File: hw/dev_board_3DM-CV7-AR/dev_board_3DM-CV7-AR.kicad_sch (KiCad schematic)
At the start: 26 parts, among them J1 87438-0643, U1 DMP2240UW, U2 DMP2240UW

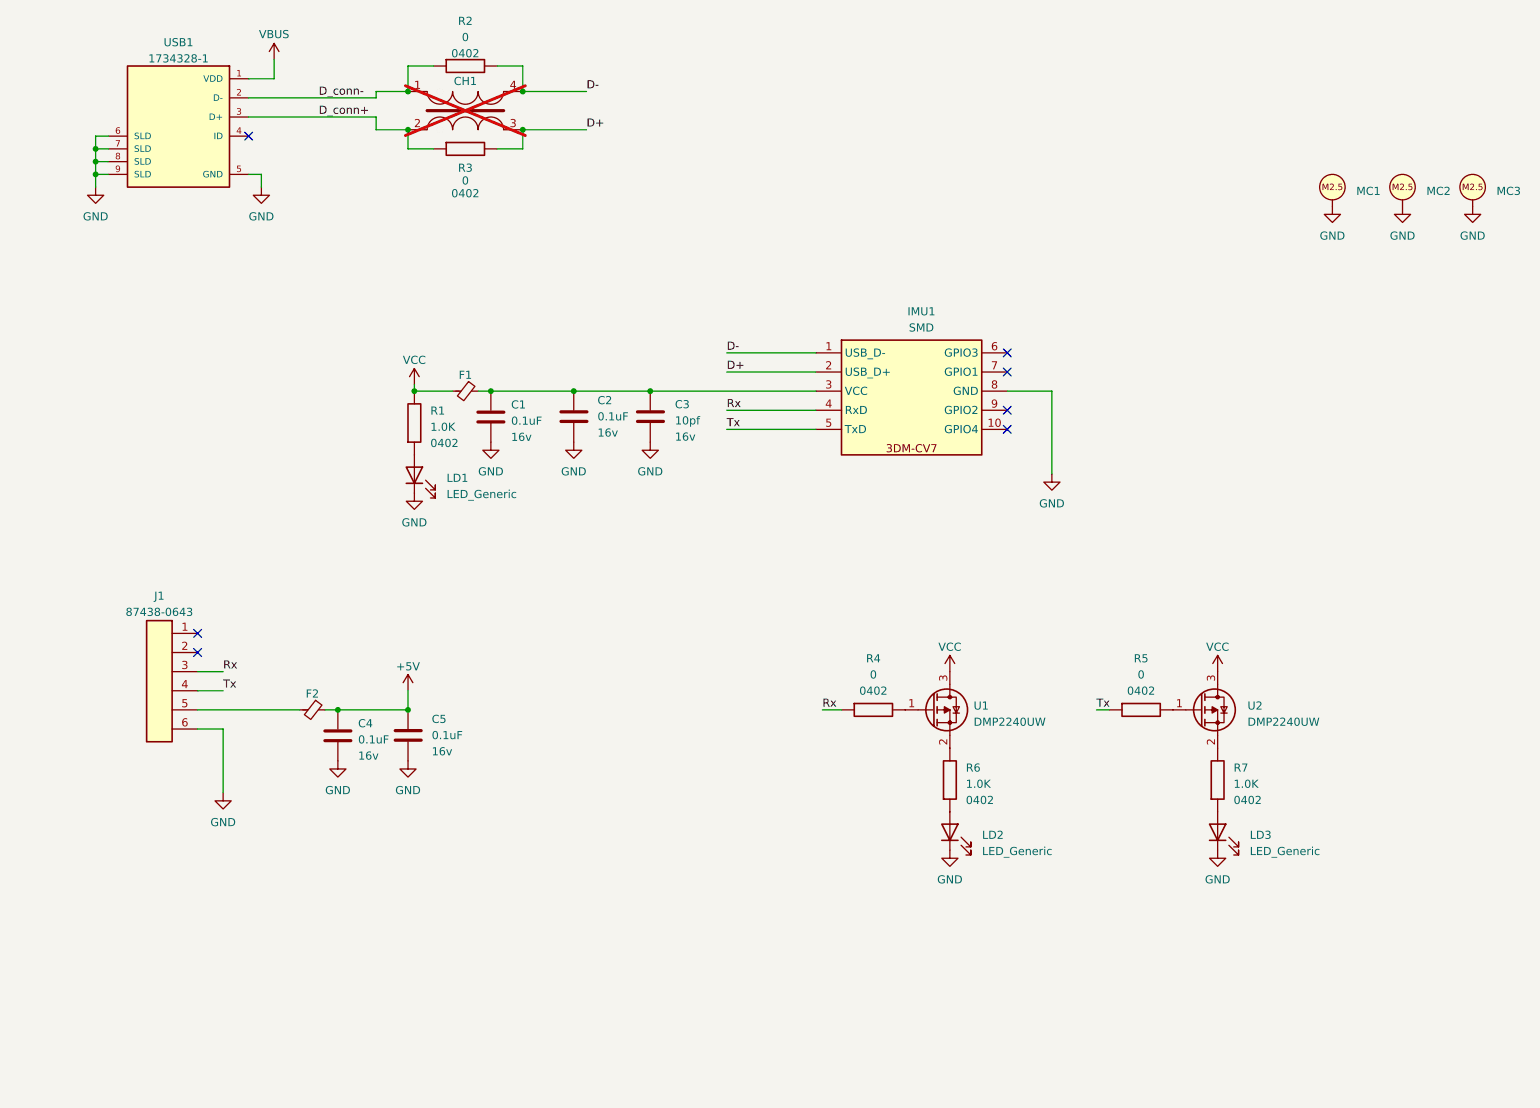
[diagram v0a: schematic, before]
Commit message: Finalizado
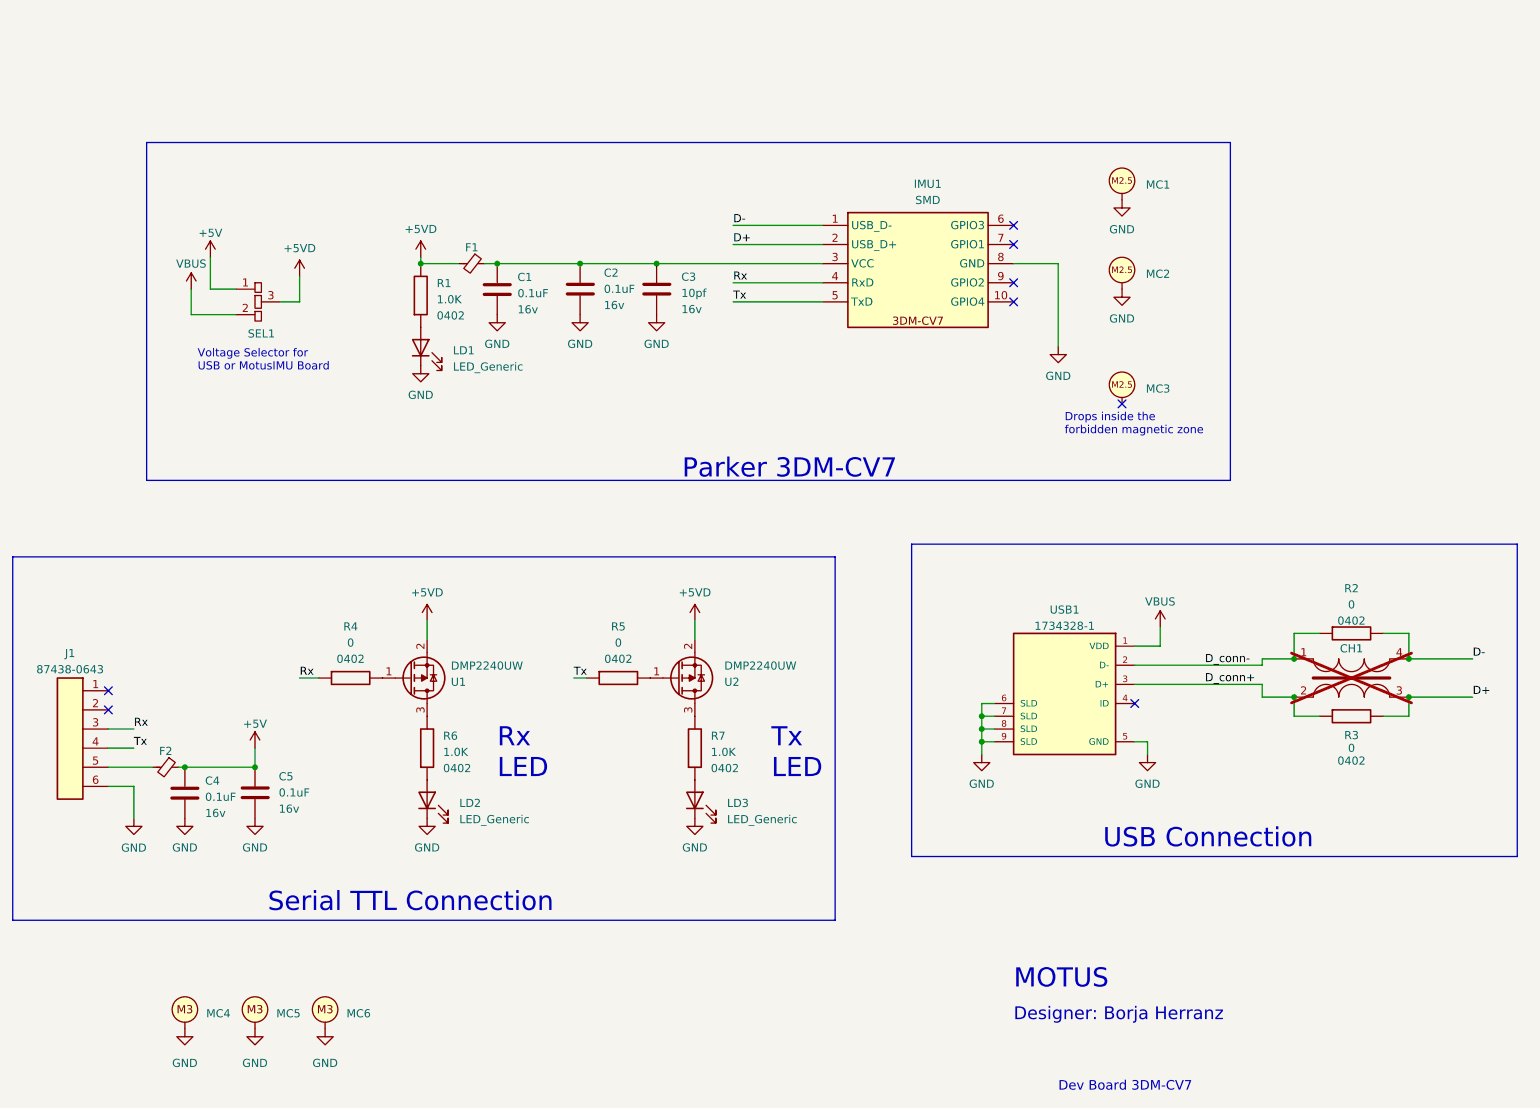
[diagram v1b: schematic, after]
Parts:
- added MC4, MC5, MC6: M3_Hole, Herranz - Various:M3_Hole, symbol Herranz - Various:M3_Hole
- added SEL1: ~, Herranz - Various:pad_selector, symbol Herranz - Various:SEL_PAD
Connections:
- net +5V: now also SEL1.1
- net GND: now also MC4.1, MC5.1, MC6.1; no longer MC3.1
- net VBUS: now also SEL1.2
- net at R6.2: now also U1.3 (D); no longer U1.2 (S)
- net at R7.2: now also U2.3 (D); no longer U2.2 (S)
- net +3V3 renamed +5VD
- net +5VD: now also U1.2 (S), U2.2 (S), SEL1.3; no longer U1.3 (D), U2.3 (D)
- no-connect marks 7 -> 8
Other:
- note added: "Designer: Borja Herranz"
- note added: "Dev Board 3DM-CV7"
- note added: "Drops inside the forbidden magnetic zone"
- note added: "MOTUS"
- note added: "Parker 3DM-CV7"
- note added: "Rx LED"
- note added: "Serial TTL Connection"
- note added: "Tx LED"
- note added: "USB Connection"
- note added: "Voltage Selector for USB or MotusIMU Board"
- moved on the sheet: C1, C2, C3, C4, C5, CH1, F1, F2, IMU1, J1, LD1, LD2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
